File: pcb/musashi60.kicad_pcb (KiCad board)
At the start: 2 copper layers, 175 x 135.7 mm, 81 parts, among them J1 MJ-4PP-9, U1 ProMicro_r

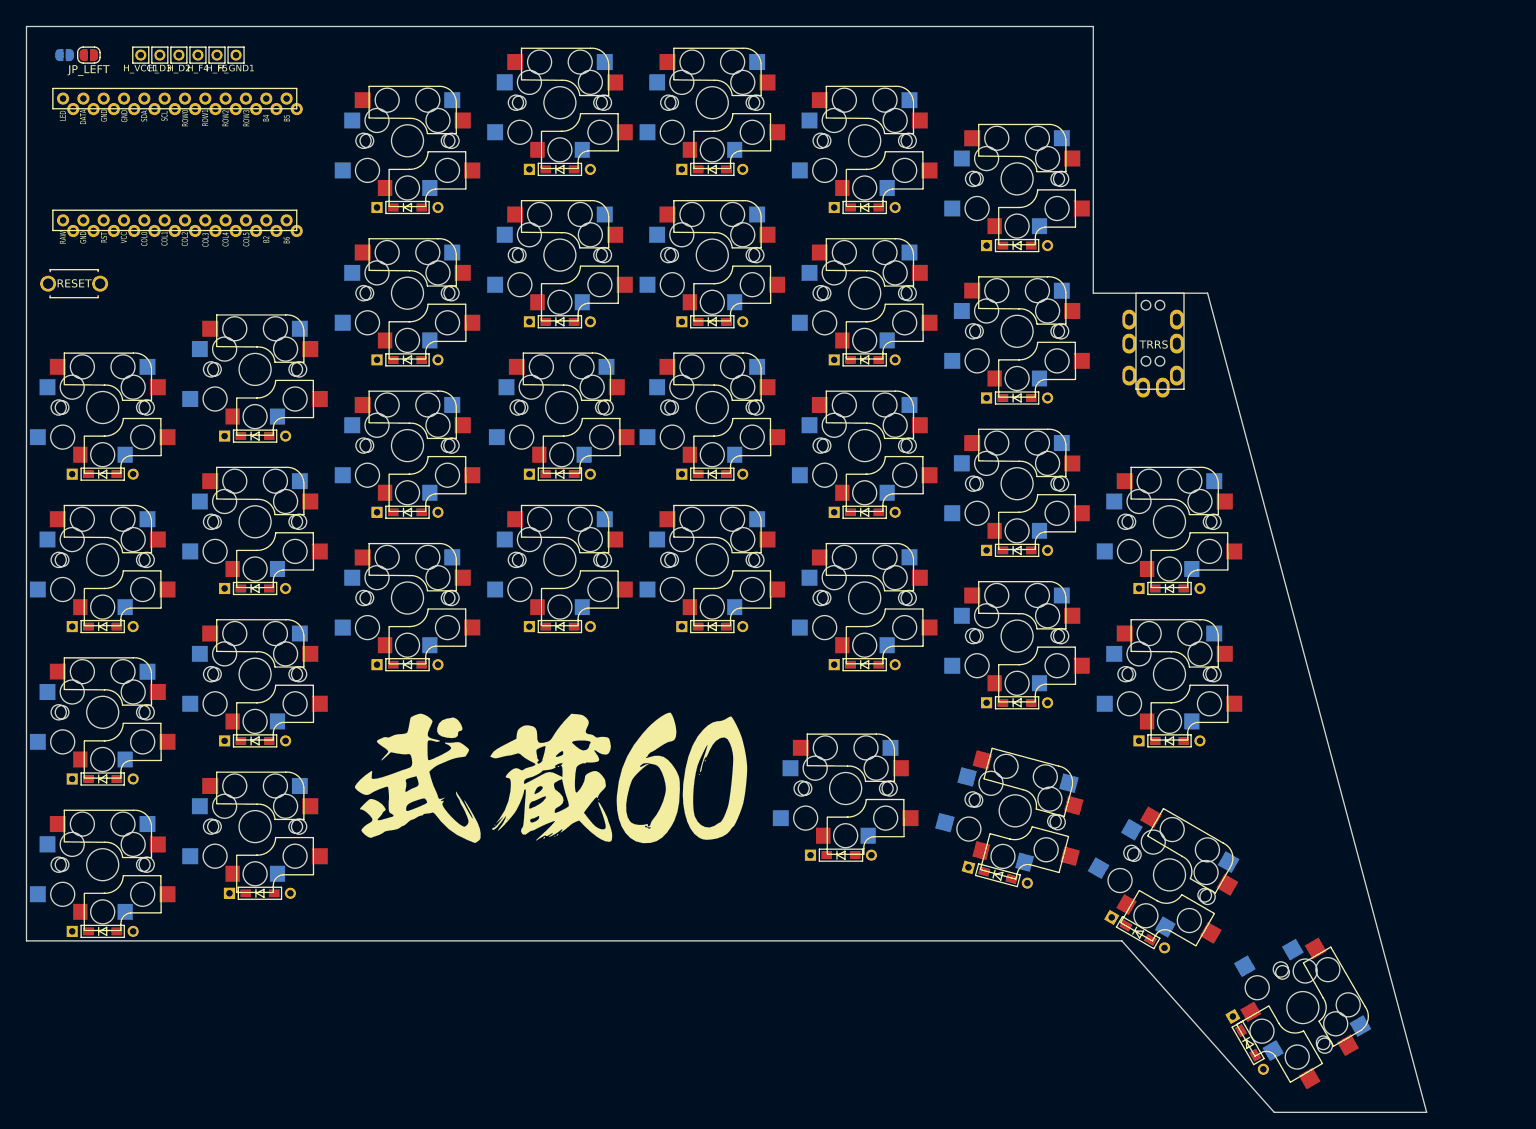
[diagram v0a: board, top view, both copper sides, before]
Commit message: update pcb
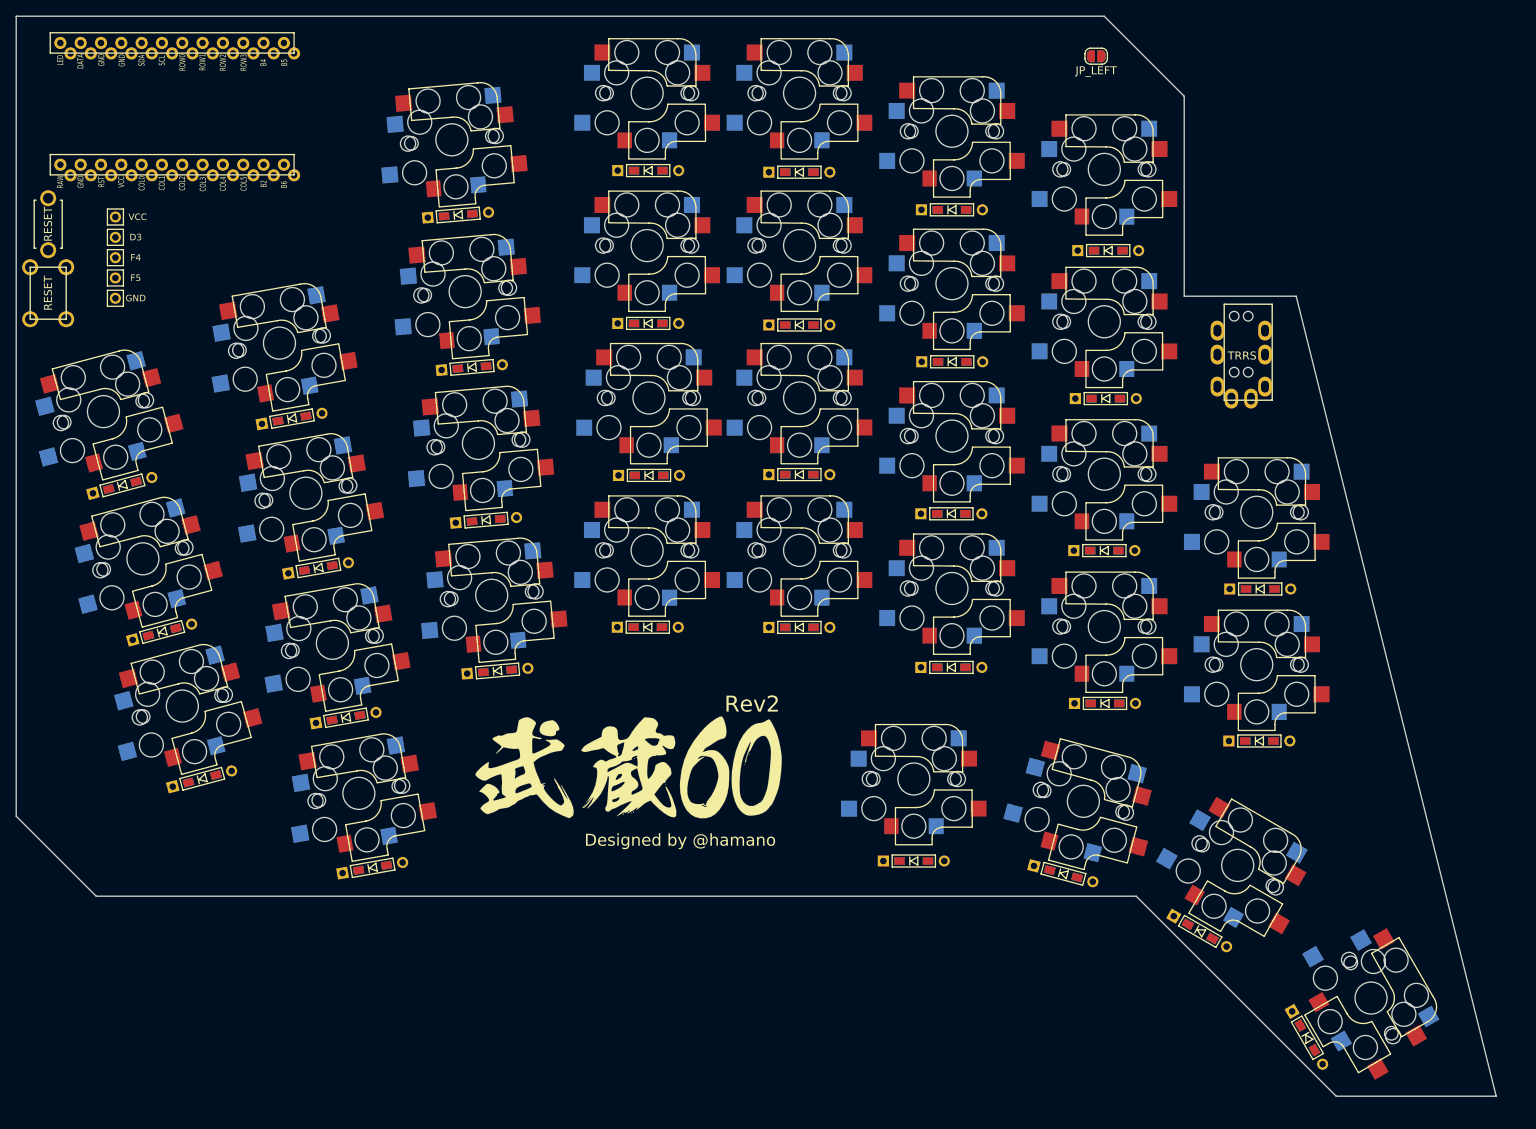
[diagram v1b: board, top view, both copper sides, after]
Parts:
- removed D_H5: D, foostan:D3_TH_SMD
- removed the G_LOGO_B at (79.8, 108.3)
- removed the G_LOGO_F at (79.8, 108.3)
- removed H_D2: MountingHole_Pad, foostan:1pin_conn
- removed SW_H5: SW_PUSH, foostan:CherryMX_Choc_Hotswap
- added G_LOGO_B: LOGO, local:musashi60-silk-256, B.Cu at (90.7, 107.0)
- added G_LOGO_F: LOGO, local:musashi60-silk-256, F.Cu at (89.5, 107.0)
- added SW_RST2: SW_PUSH, foostan:ResetSW_4P, F.Cu at (17.0, 47.6)
- moved JP_RIGHT 128.9 mm to (148.0, 18.0)
- moved JP_LEFT 125.9 mm to (148.0, 18.0)
- moved GND 33.9 mm to (25.4, 48.3)
- moved F5 30.6 mm to (25.4, 45.7)
- moved F4 27.3 mm to (25.4, 43.2)
- moved D3 23.4 mm to (25.4, 40.6)
- moved VCC 20.5 mm to (25.4, 38.1)
- moved D_G5 14.4 mm to (57.5, 119.5), turned to 10 degrees
- moved SW_G5 13.6 mm to (55.8, 110.1), turned to 10 degrees
- moved D_H4 12.4 mm to (36.2, 108.3), turned to 15 degrees
- moved D_G4 11.7 mm to (54.2, 100.7), turned to 10 degrees
- moved D_B1 11.4 mm to (149.5, 42.3)
- moved D_A3 11.3 mm to (168.5, 84.6)
- moved D_F4 11.3 mm to (73.2, 94.8), turned to 5 degrees
- moved D_A4 11.2 mm to (168.4, 103.6)
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- renumbered H_D3 to D3, H_F4 to F4, H_F5 to F5, H_GND1 to GND, H_VCC1 to VCC
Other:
- board size 175 x 135.7 mm -> 185 x 135 mm
- board text added: "Designed by @hamano"
- board text added: "Rev2"

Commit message: update pcb
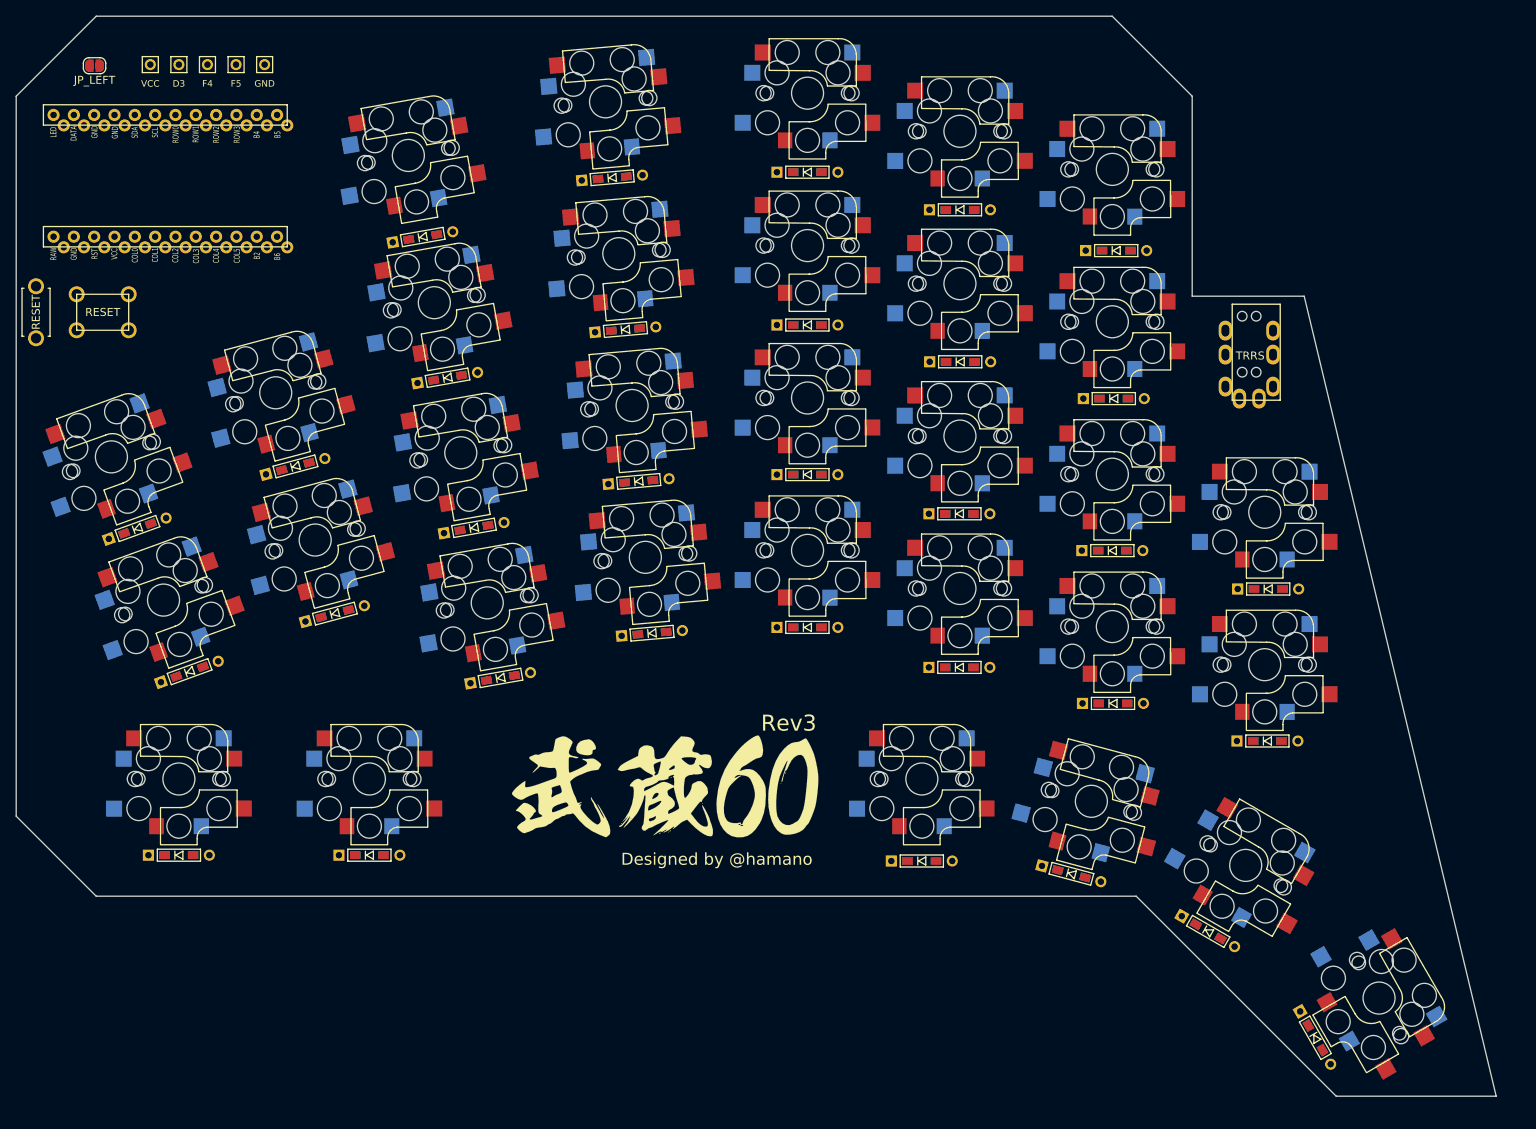
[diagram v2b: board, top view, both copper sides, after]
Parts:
- removed D_G5: D, foostan:D3_TH_SMD
- removed SW_G5: SW_PUSH, foostan:CherryMX_Choc_Hotswap
- moved JP_LEFT 125.2 mm to (22.8, 19.2)
- moved JP_RIGHT 125.2 mm to (22.8, 19.2)
- moved GND 34.7 mm to (44.1, 19.1)
- moved F5 30.6 mm to (40.5, 19.1)
- moved F4 26.7 mm to (36.9, 19.1)
- moved D3 23.0 mm to (33.3, 19.1)
- moved VCC 19.5 mm to (29.8, 19.1)
- moved SW_G4 17.6 mm to (57.2, 108.3), turned to 0 degrees
- moved D_G4 17.4 mm to (57.2, 117.9), turned to 0 degrees
- moved SW_RST1 11.1 mm to (15.5, 50.0)
- moved D_H4 9.98 mm to (33.3, 117.9), turned to 0 degrees
- moved SW_H4 9.13 mm to (33.3, 108.3), turned to 0 degrees
- moved U1 9.04 mm to (32.1, 33.0)
- moved SW_RST2 7.22 mm to (23.8, 50.0), turned to 180 degrees
- moved SW_G2 6.23 mm to (45.4, 60.1), turned to 15 degrees
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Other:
- outline, holes or cut-outs redrawn
- board text added: "Rev3"
- board text removed: "Rev2"

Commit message: update pcb
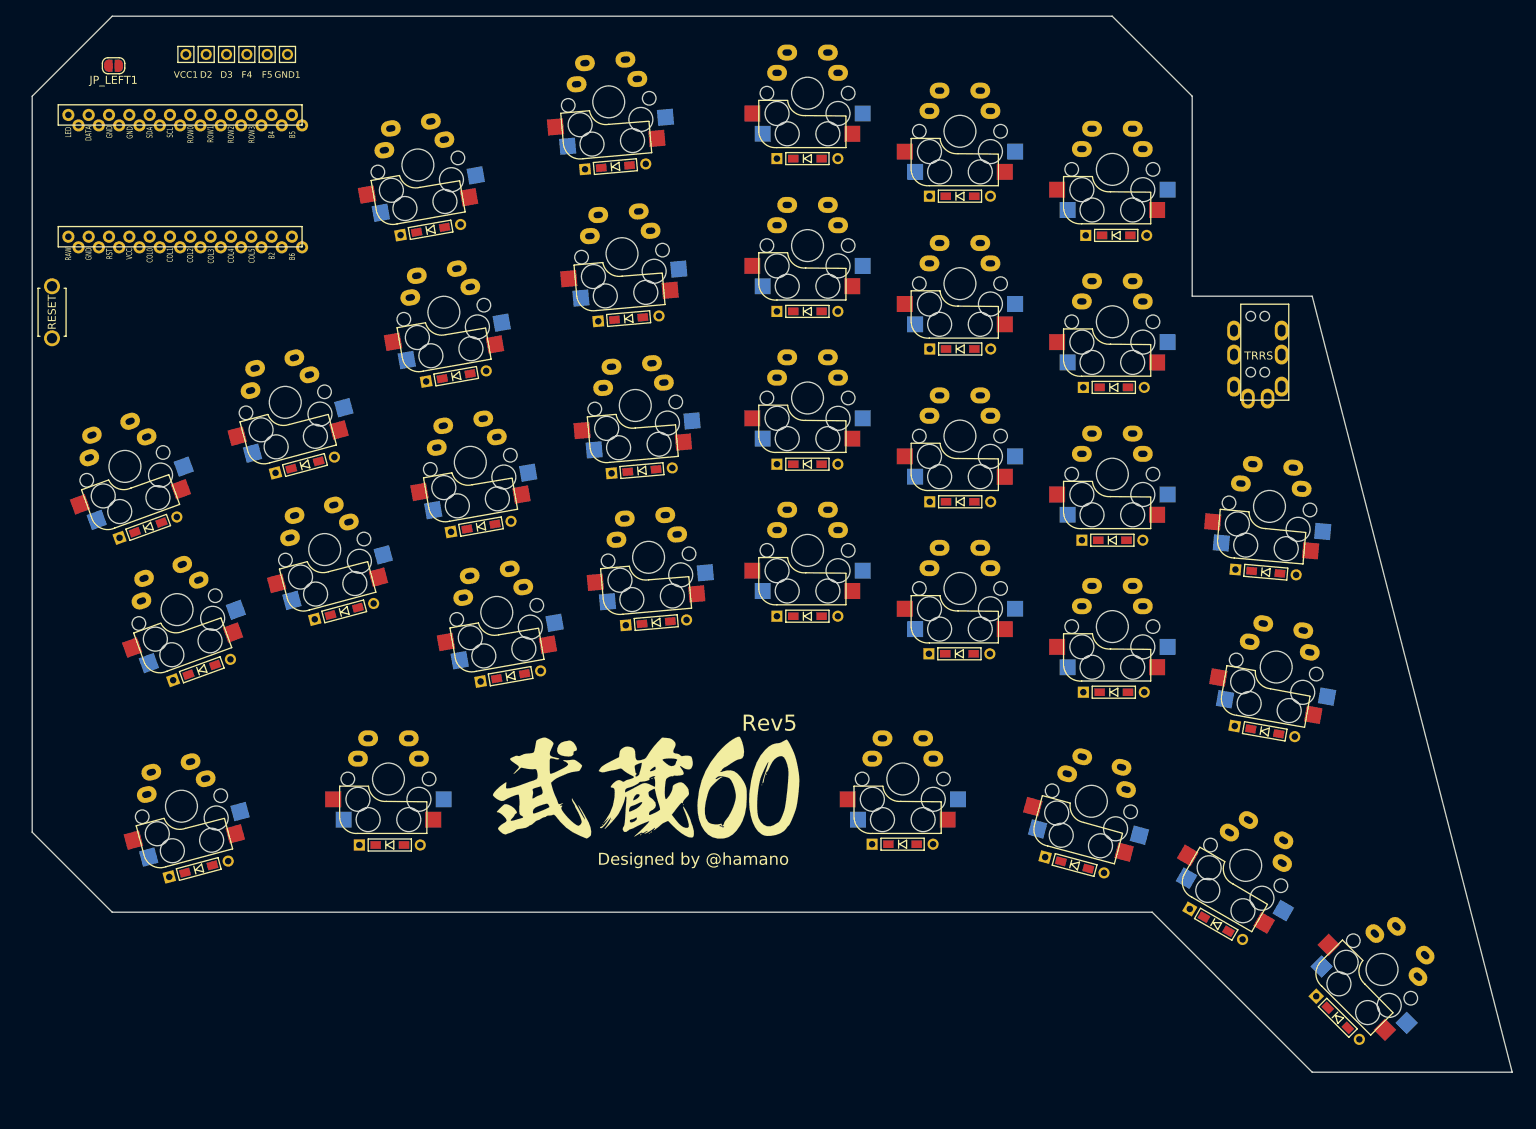
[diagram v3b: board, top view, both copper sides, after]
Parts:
- removed JP_LEFT: Jumper, Jumper:SolderJumper-2_P1.3mm_Open_RoundedPad1.0x1.5mm
- removed SW_RST2: SW_PUSH, foostan:ResetSW_4P
- added D2: MountingHole_Pad, foostan:1pin_conn, F.Cu at (36.8, 17.8)
- added JP_LEFT1: Jumper, Jumper:SolderJumper-2_P1.3mm_Open_RoundedPad1.0x1.5mm, F.Cu at (25.2, 19.2)
- SW_A3, SW_A4, SW_A5, SW_B1, SW_B2, SW_B3, SW_B4, SW_B5, SW_C1, SW_C2, SW_C3, SW_C4, SW_C5, SW_D1, SW_D2, SW_D3, SW_D4, SW_D5, SW_E1, SW_E2, SW_E3, SW_E4, SW_F1, SW_F2, SW_F3, SW_F4, SW_G2, SW_G3, SW_G4, SW_H2, SW_H3, SW_H4: footprint foostan:CherryMX_Choc_Hotswap -> local:CherryMX_Direct_Hotswap_Reversible
- moved D3 6.09 mm to (39.3, 17.8)
- moved F4 5.08 mm to (41.8, 17.8)
- moved VCC1 4.62 mm to (34.2, 17.8)
- moved F5 4.09 mm to (44.4, 17.8)
- moved D_A5 3.75 mm to (178.2, 138.2), turned to 315 degrees
- moved SW_A5 3.59 mm to (183.7, 132.2), turned to 315 degrees
- moved SW_H4 3.42 mm to (33.7, 111.8), turned to 15 degrees
- moved D_D5 3.19 mm to (123.8, 116.5)
- moved GND1 3.13 mm to (46.9, 17.8)
- moved D_H4 3.02 mm to (35.8, 119.6), turned to 15 degrees
- moved D_G4 2.85 mm to (59.7, 116.6)
- moved G_LOGO_F 2.39 mm to (91.7, 109.5)
- moved SW_G4 2.38 mm to (59.5, 108.3)
- moved JP_RIGHT1 2.38 mm to (25.2, 19.2)
- moved SW_D5 2.38 mm to (123.8, 108.3)
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- renumbered GND to GND1, JP_RIGHT to JP_RIGHT1, VCC to VCC1
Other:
- board size 185 x 135 mm -> 185 x 132 mm
- board text added: "Rev5"
- board text removed: "Rev3"
